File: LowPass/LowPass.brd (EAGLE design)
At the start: 50.8 x 17.4 mm, 10 parts

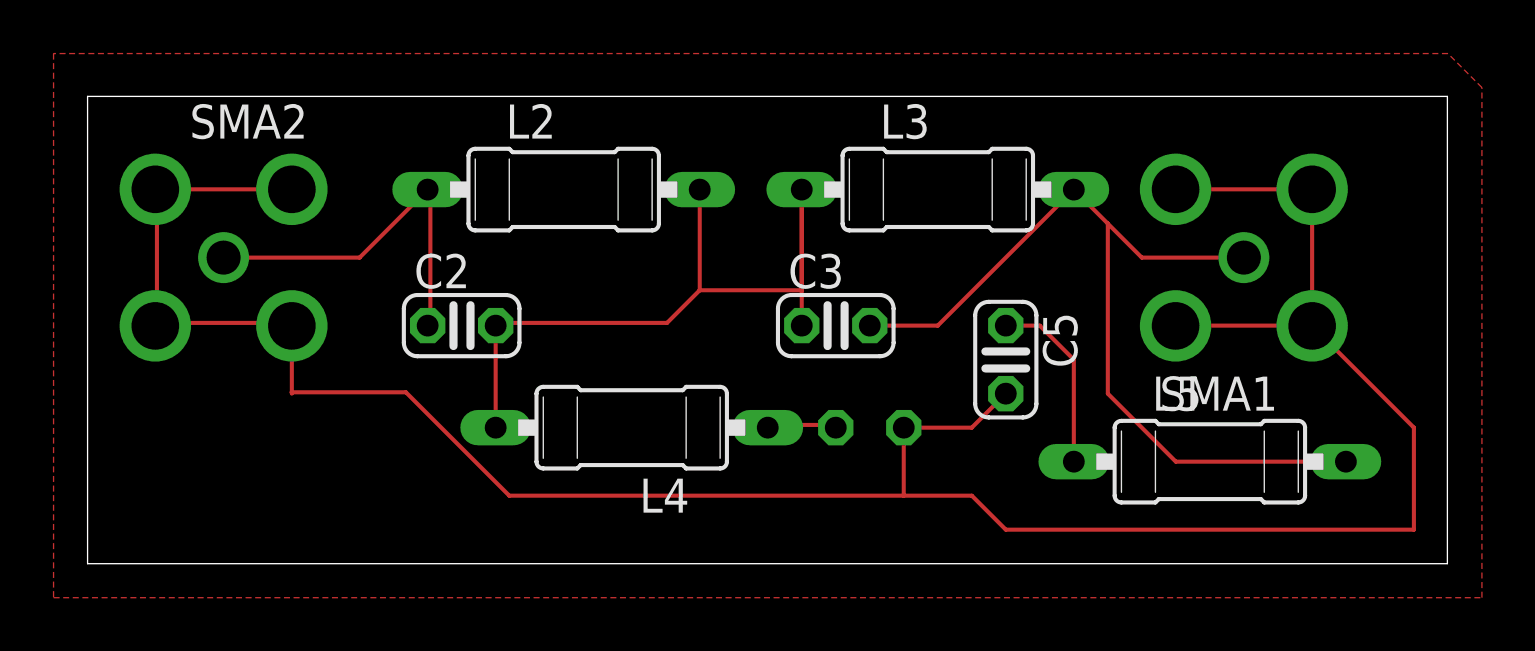
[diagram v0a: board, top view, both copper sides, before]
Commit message: Update PCB
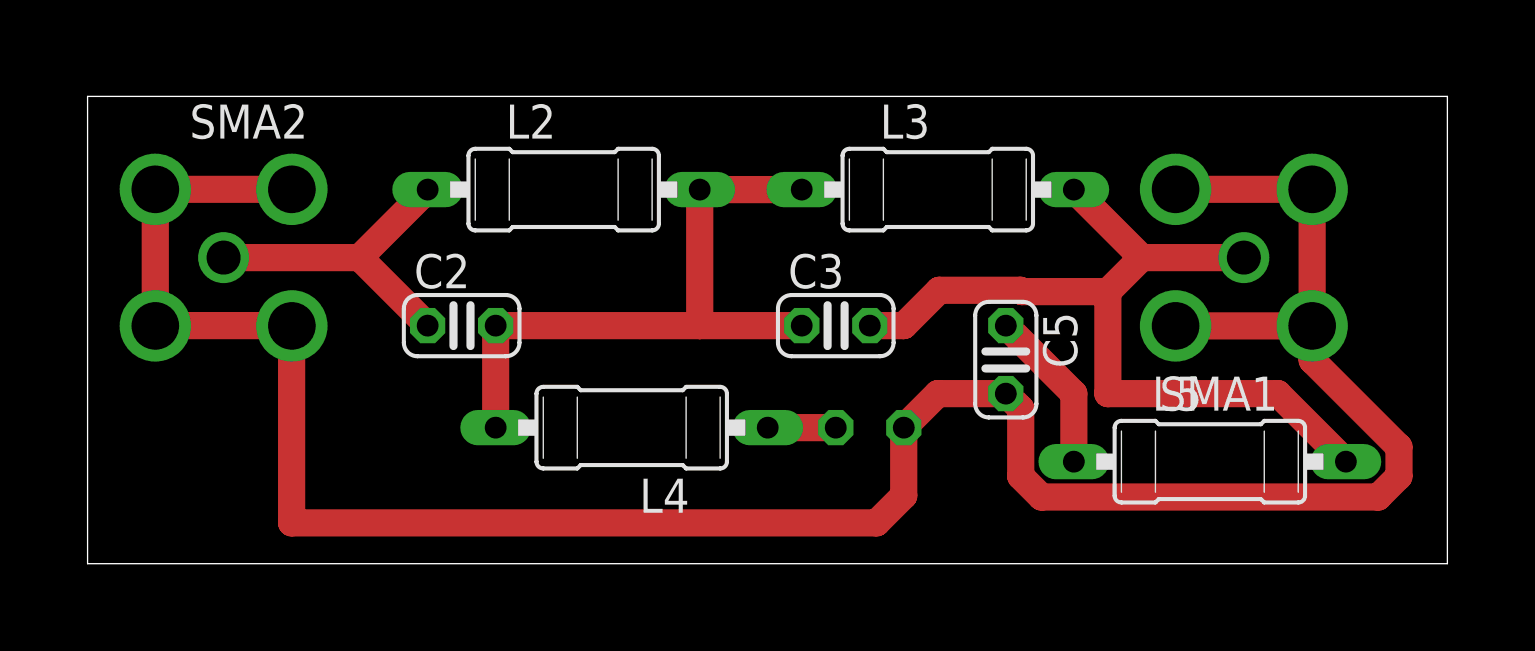
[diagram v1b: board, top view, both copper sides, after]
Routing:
- net N$5: track 28.4 -> 24.2 mm
- net N$3: track 13.9 -> 12.3 mm
- net N$7: track 33.5 -> 32.5 mm
- net N$9: track 6.88 -> 6.13 mm
- removed copper zone on layer 1, net GND
